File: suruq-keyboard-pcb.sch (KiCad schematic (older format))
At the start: 20 parts, among them J1 AVR-ISP-6, SW65 SW_Push, U1 PRTR5V0U2X, U2 ATmega32U4-AU, Y1 16MHz

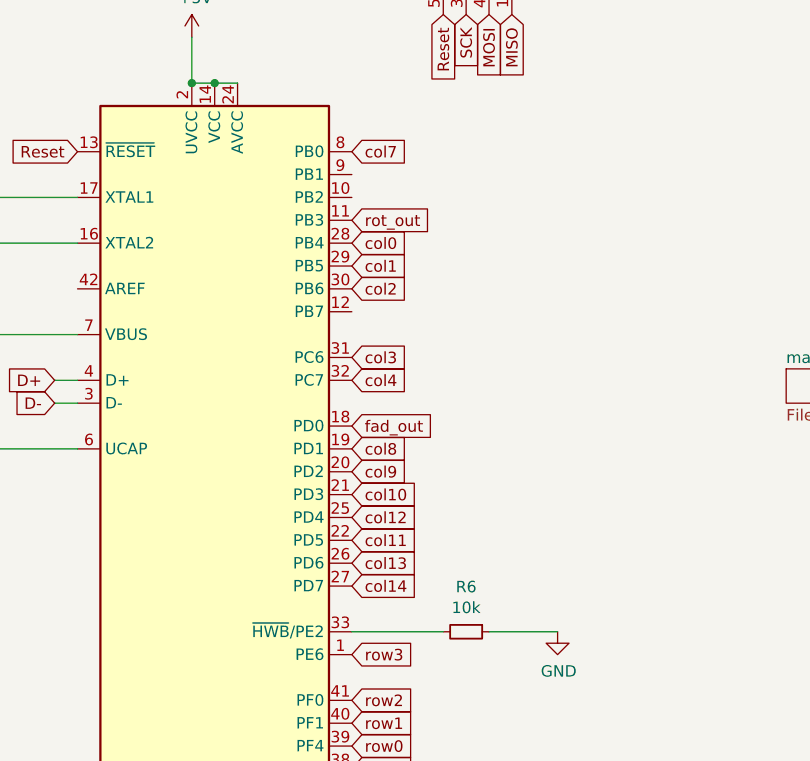
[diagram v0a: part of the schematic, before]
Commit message: fin routing
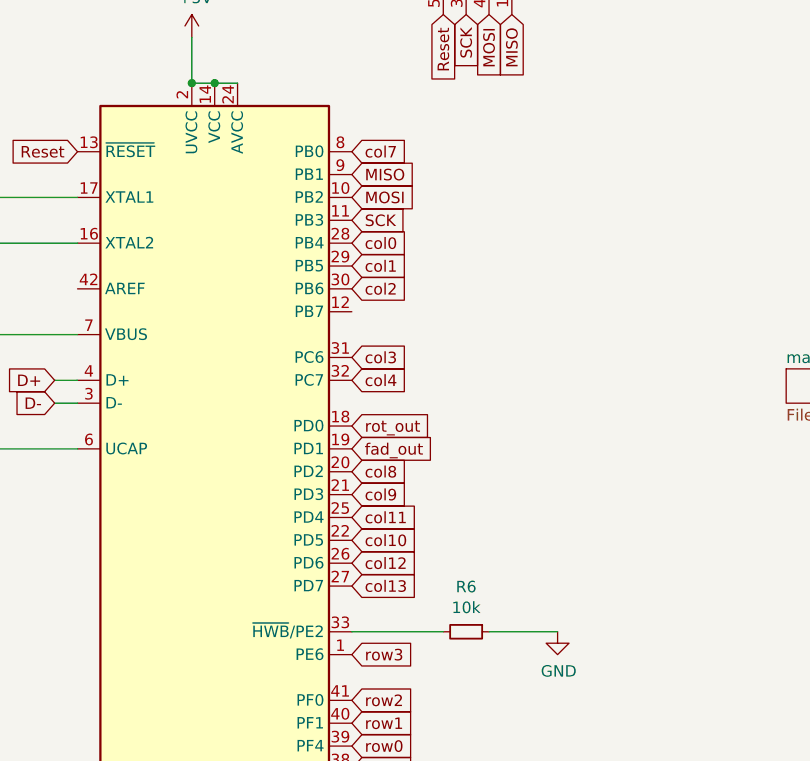
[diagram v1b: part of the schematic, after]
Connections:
- net col14 is gone; now on net col13: U2.27 (PD7)
- net MISO: now also U2.9 (PB1)
- net MOSI: now also U2.10 (PB2)
- net SCK: now also U2.11 (PB3)
- net col10: now also U2.22 (PD5); no longer U2.21 (PD3)
- net col11: now also U2.25 (PD4); no longer U2.22 (PD5)
- net col12: now also U2.26 (PD6); no longer U2.25 (PD4)
- net col13: no longer U2.26 (PD6)
- net col8: now also U2.20 (PD2); no longer U2.19 (PD1)
- net col9: now also U2.21 (PD3); no longer U2.20 (PD2)
- net fad_out: now also U2.19 (PD1); no longer U2.18 (PD0)
- net rot_out: now also U2.18 (PD0); no longer U2.11 (PB3)
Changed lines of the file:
@@
 Text GLabel 7400 1750 3    50   Input ~ 0
 MISO
-Text GLabel 7300 1750 3    50   Input ~ 0
-MOSI
 Text GLabel 7200 1750 3    50   Input ~ 0
 SCK
@@
 Text GLabel 6700 3350 2    50   Input ~ 0
 col4
-Text GLabel 6700 3650 2    50   Input ~ 0
+Text GLabel 6700 3750 2    50   Input ~ 0
 col8
-Text GLabel 6700 3750 2    50   Input ~ 0
+Text GLabel 6700 3850 2    50   Input ~ 0
 col9
-Text GLabel 6700 3850 2    50   Input ~ 0
+Text GLabel 6700 4050 2    50   Input ~ 0
 col10
+Text GLabel 6700 4150 2    50   Input ~ 0
+col12
 Text GLabel 6700 3950 2    50   Input ~ 0
-col12
-Text GLabel 6700 4050 2    50   Input ~ 0
 col11
-Text GLabel 6700 4150 2    50   Input ~ 0
+Text GLabel 6700 4250 2    50   Input ~ 0
 col13
-Text GLabel 6700 4250 2    50   Input ~ 0
-col14
 Text GLabel 6700 4950 2    50   Input ~ 0
 row0
@@
 Text GLabel 6700 5150 2    50   Input ~ 0
 col6
+Text GLabel 6700 3650 2    50   Input ~ 0
+fad_out
 Text GLabel 6700 3550 2    50   Input ~ 0
-fad_out
-Text GLabel 6700 2650 2    50   Input ~ 0
 rot_out
 $Comp
@@
 Text GLabel 2100 3450 1    50   Input ~ 0
 DN
+Text GLabel 6700 2650 2    50   Input ~ 0
+SCK
+Text GLabel 7300 1750 3    50   Input ~ 0
+MOSI
+Text GLabel 6700 2550 2    50   Input ~ 0
+MOSI
+Text GLabel 6700 2450 2    50   Input ~ 0
+MISO
 $EndSCHEMATC
